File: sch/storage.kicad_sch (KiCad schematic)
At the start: 9 parts, among them U3 74HC126

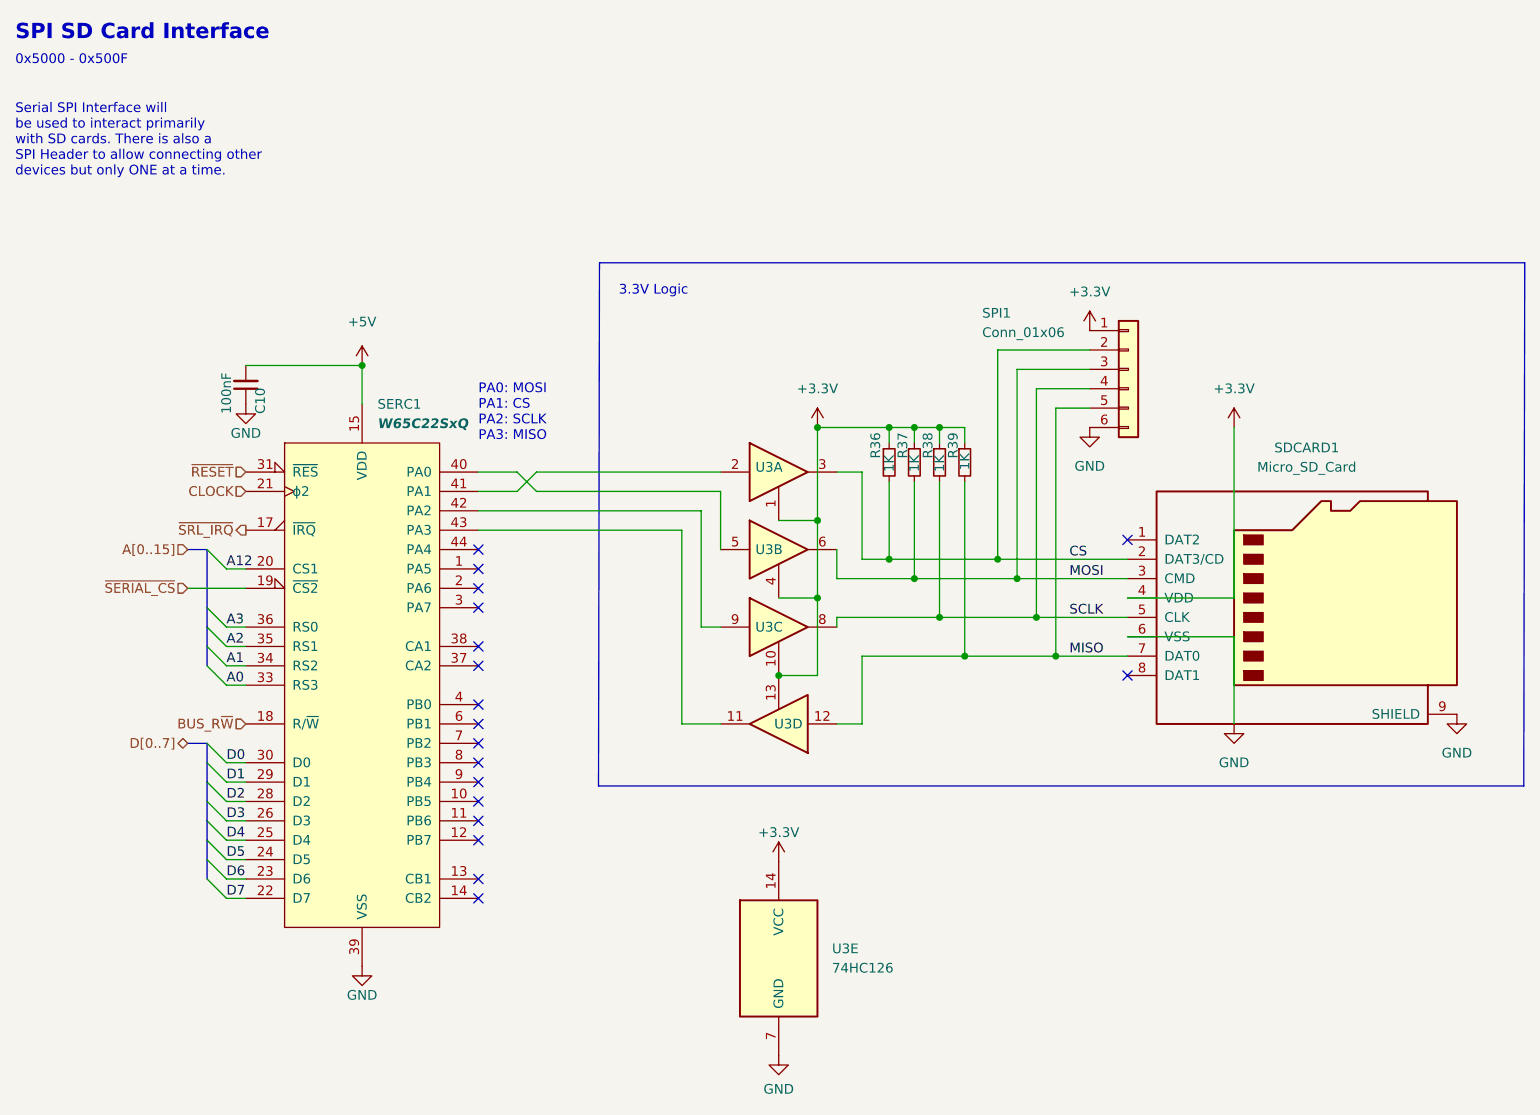
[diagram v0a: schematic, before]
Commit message: improve routing
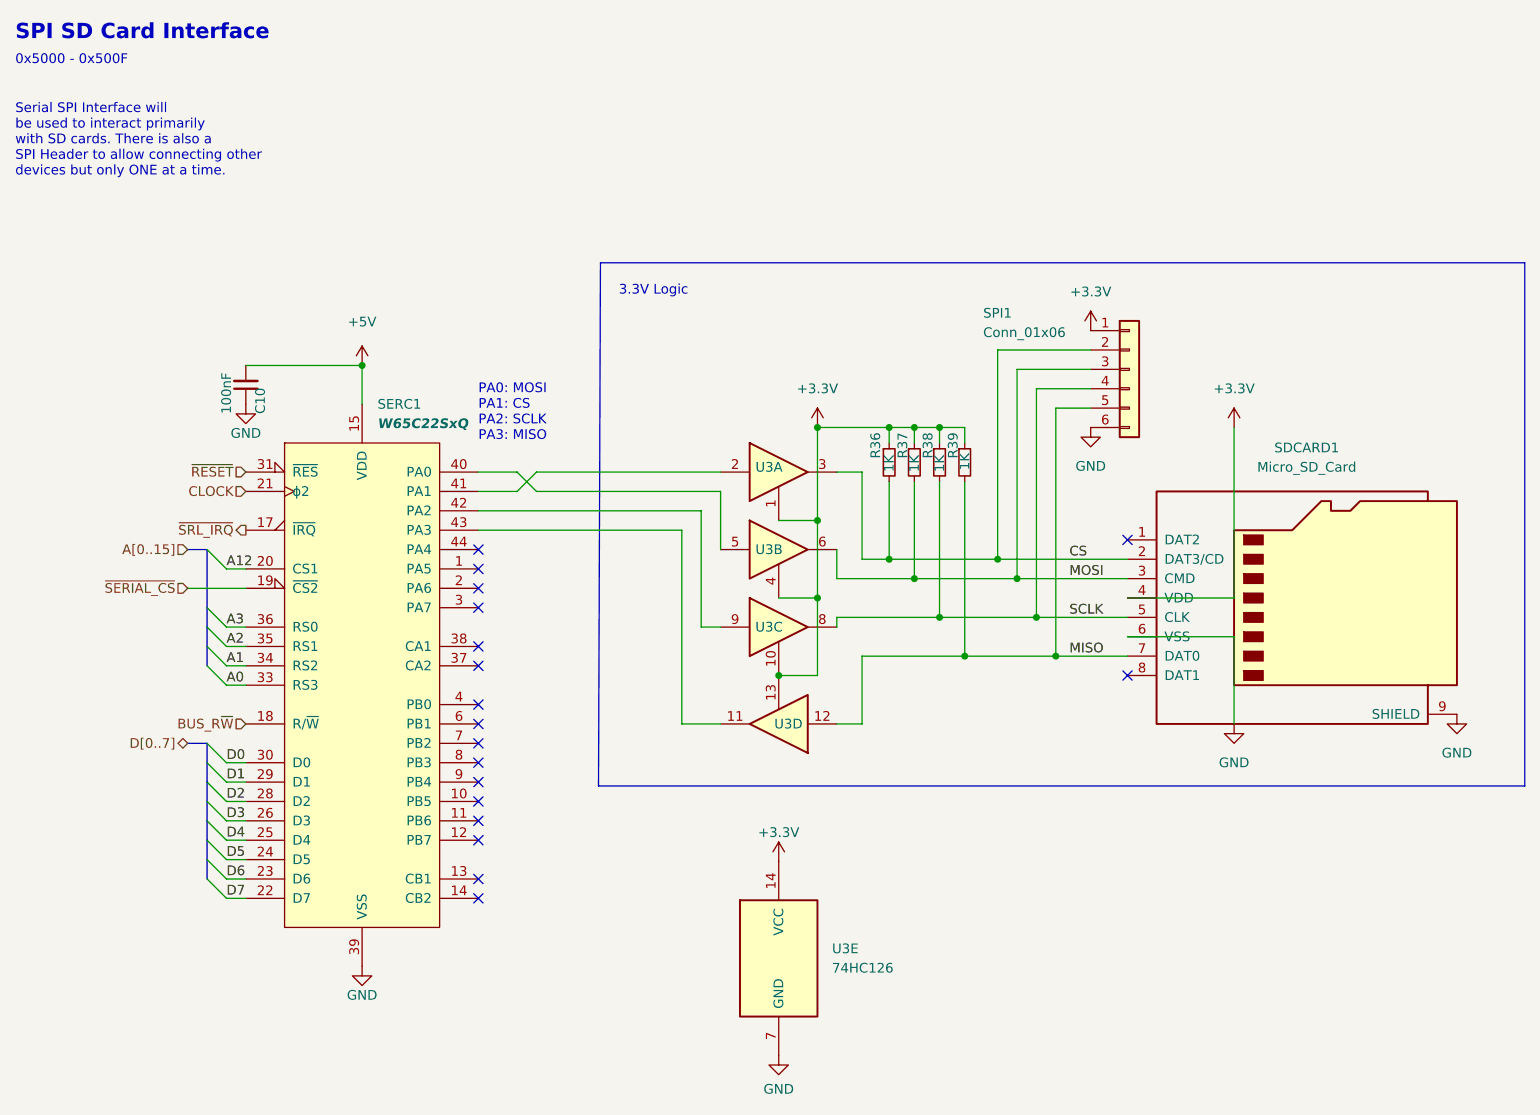
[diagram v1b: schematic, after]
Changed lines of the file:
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@@
     (stroke (width 0) (type default) (color 0 0 0 0))
   )
-  (wire (pts (xy 166.243 68.326) (xy 154.178 68.326))
+  (wire (pts (xy 166.37 68.326) (xy 154.178 68.326))
     (stroke (width 0) (type default) (color 0 0 0 0))
   )
@@
     (stroke (width 0) (type default) (color 0 0 0 0))
   )
-  (wire (pts (xy 166.243 73.406) (xy 159.258 73.406))
+  (wire (pts (xy 166.37 73.406) (xy 159.258 73.406))
     (stroke (width 0) (type default) (color 0 0 0 0))
   )
@@
     (stroke (width 0) (type default) (color 0 0 0 0))
   )
-  (polyline (pts (xy 101.981 56.896) (xy 223.266 56.896))
+  (polyline (pts (xy 102.108 56.896) (xy 223.266 56.896))
     (stroke (width 0) (type default) (color 0 0 0 0))
   )
@@
     (stroke (width 0) (type default) (color 0 0 0 0))
   )
-  (polyline (pts (xy 101.981 56.896) (xy 101.854 125.476))
+  (polyline (pts (xy 102.108 56.896) (xy 101.854 125.476))
     (stroke (width 0) (type default) (color 0 0 0 0))
   )
@@
     (stroke (width 0) (type default) (color 0 0 0 0))
   )
-  (polyline (pts (xy 223.139 125.476) (xy 223.266 56.896))
+  (polyline (pts (xy 223.266 125.476) (xy 223.266 56.896))
     (stroke (width 0) (type default) (color 0 0 0 0))
   )
@@
     (stroke (width 0) (type default) (color 0 0 0 0))
   )
-  (polyline (pts (xy 101.854 125.476) (xy 223.139 125.476))
-    (stroke (width 0) (type default) (color 0 0 0 0))
-  )
-  (wire (pts (xy 166.243 75.946) (xy 161.798 75.946))
+  (polyline (pts (xy 101.854 125.476) (xy 223.266 125.476))
+    (stroke (width 0) (type default) (color 0 0 0 0))
+  )
+  (wire (pts (xy 166.37 75.946) (xy 161.798 75.946))
     (stroke (width 0) (type default) (color 0 0 0 0))
   )
@@
     (stroke (width 0) (type default) (color 0 0 0 0))
   )
-  (wire (pts (xy 166.243 70.866) (xy 156.718 70.866))
+  (wire (pts (xy 166.37 70.866) (xy 156.718 70.866))
     (stroke (width 0) (type default) (color 0 0 0 0))
   )
@@
     (pin "1")
   )
-  (symbol (lib_id "power:GND") (at 166.243 78.486 0) (unit 1)
-    (in_bom yes) (on_board yes) (fields_autoplaced)
-    (property "Reference" "#PWR0109" (id 0) (at 166.243 84.836 0)
-      (effects (font (size 1.27 1.27)) hide)
-    )
-    (property "Value" "GND" (id 1) (at 166.243 83.566 0))
-    (property "Footprint" "" (id 2) (at 166.243 78.486 0)
-      (effects (font (size 1.27 1.27)) hide)
-    )
-    (property "Datasheet" "" (id 3) (at 166.243 78.486 0)
+  (symbol (lib_id "power:GND") (at 166.37 78.486 0) (unit 1)
+    (in_bom yes) (on_board yes) (fields_autoplaced)
+    (property "Reference" "#PWR0109" (id 0) (at 166.37 84.836 0)
+      (effects (font (size 1.27 1.27)) hide)
+    )
+    (property "Value" "GND" (id 1) (at 166.37 83.566 0))
+    (property "Footprint" "" (id 2) (at 166.37 78.486 0)
+      (effects (font (size 1.27 1.27)) hide)
+    )
+    (property "Datasheet" "" (id 3) (at 166.37 78.486 0)
       (effects (font (size 1.27 1.27)) hide)
     )
@@
     (pin "7")
   )
-  (symbol (lib_id "Connector_Generic:Conn_01x06") (at 171.323 70.866 0) (unit 1)
-    (in_bom yes) (on_board yes)
-    (property "Reference" "SPI1" (id 0) (at 152.146 63.5 0)
-      (effects (font (size 1.27 1.27)) (justify left))
-    )
-    (property "Value" "Conn_01x06" (id 1) (at 152.146 66.04 0)
-      (effects (font (size 1.27 1.27)) (justify left))
-    )
-    (property "Footprint" "Connector_PinHeader_2.54mm:PinHeader_1x06_P2.54mm_Vertical" (id 2) (at 171.323 70.866 0)
-      (effects (font (size 1.27 1.27)) hide)
-    )
-    (property "Datasheet" "~" (id 3) (at 171.323 70.866 0)
+  (symbol (lib_id "Connector_Generic:Conn_01x06") (at 171.45 70.866 0) (unit 1)
+    (in_bom yes) (on_board yes)
+    (property "Reference" "SPI1" (id 0) (at 152.273 63.5 0)
+      (effects (font (size 1.27 1.27)) (justify left))
+    )
+    (property "Value" "Conn_01x06" (id 1) (at 152.273 66.04 0)
+      (effects (font (size 1.27 1.27)) (justify left))
+    )
+    (property "Footprint" "Connector_PinHeader_2.54mm:PinHeader_1x06_P2.54mm_Vertical" (id 2) (at 171.45 70.866 0)
+      (effects (font (size 1.27 1.27)) hide)
+    )
+    (property "Datasheet" "~" (id 3) (at 171.45 70.866 0)
       (effects (font (size 1.27 1.27)) hide)
     )
@@
     (pin "7")
   )
-  (symbol (lib_id "power:+3.3V") (at 166.243 65.786 0) (unit 1)
-    (in_bom yes) (on_board yes) (fields_autoplaced)
-    (property "Reference" "#PWR0108" (id 0) (at 166.243 69.596 0)
-      (effects (font (size 1.27 1.27)) hide)
-    )
-    (property "Value" "+3.3V" (id 1) (at 166.243 60.706 0))
-    (property "Footprint" "" (id 2) (at 166.243 65.786 0)
-      (effects (font (size 1.27 1.27)) hide)
-    )
-    (property "Datasheet" "" (id 3) (at 166.243 65.786 0)
-      (effects (font (size 1.27 1.27)) hide)
-    )
+  (symbol (lib_id "power:+3.3V") (at 166.37 65.786 0) (unit 1)
+    (in_bom yes) (on_board yes) (fields_autoplaced)
+    (property "Reference" "#PWR0108" (id 0) (at 166.37 69.596 0)
+      (effects (font (size 1.27 1.27)) hide)
+    )
+    (property "Value" "+3.3V" (id 1) (at 166.37 60.706 0))
+    (property "Footprint" "" (id 2) (at 166.37 65.786 0)
+      (effects (font (size 1.27 1.27)) hide)
+    )
+    (property "Datasheet" "" (id 3) (at 166.37 65.786 0)
+      (effects (font (size 1.27 1.27)) hide)
+    )
